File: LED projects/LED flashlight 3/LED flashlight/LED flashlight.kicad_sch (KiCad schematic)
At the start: 14 parts, among them P1 USB_C_Plug_USB2.0, SW1 SW_Push, U1 TP4056

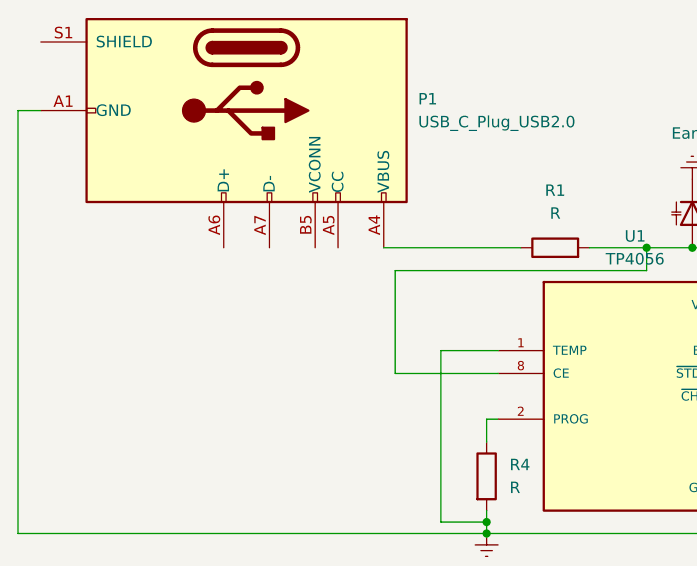
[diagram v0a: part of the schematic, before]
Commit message: update
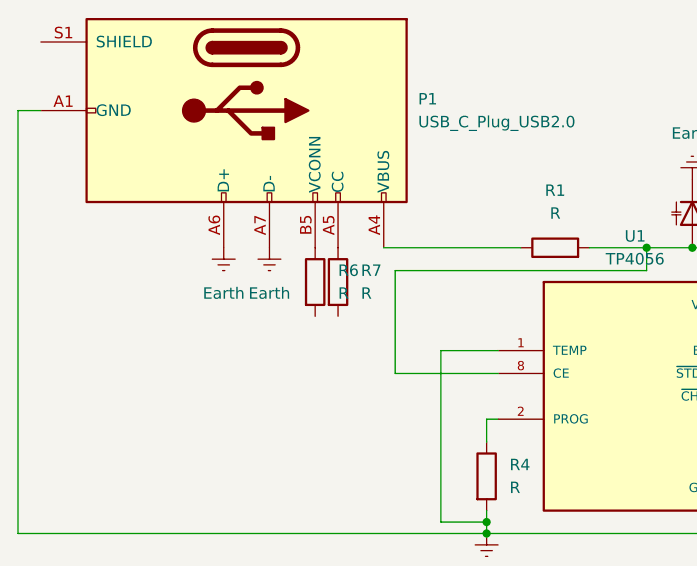
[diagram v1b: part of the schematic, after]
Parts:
- added R6, R7: R, symbol Device:R
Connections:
- net Earth: now also P1.A6 (D+), P1.A7 (D-)
- net at P1.A5 (CC): now also R7.1
- net at P1.B5 (VCONN): now also R6.1

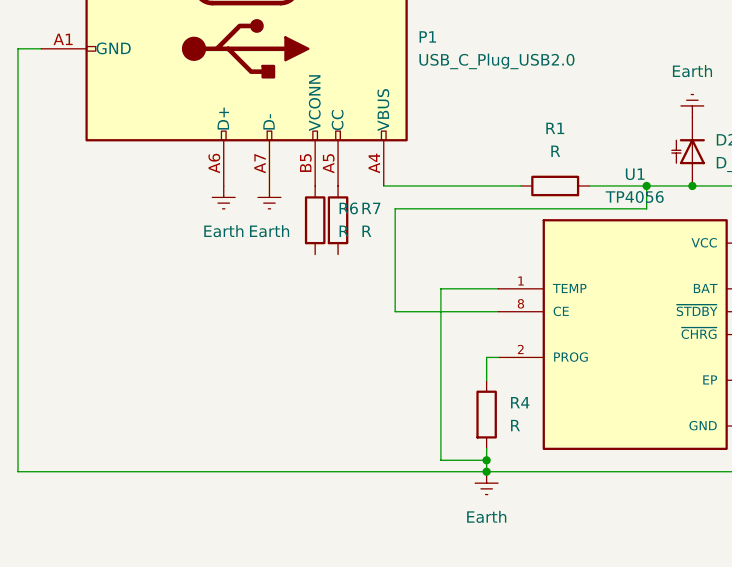
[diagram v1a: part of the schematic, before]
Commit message: update
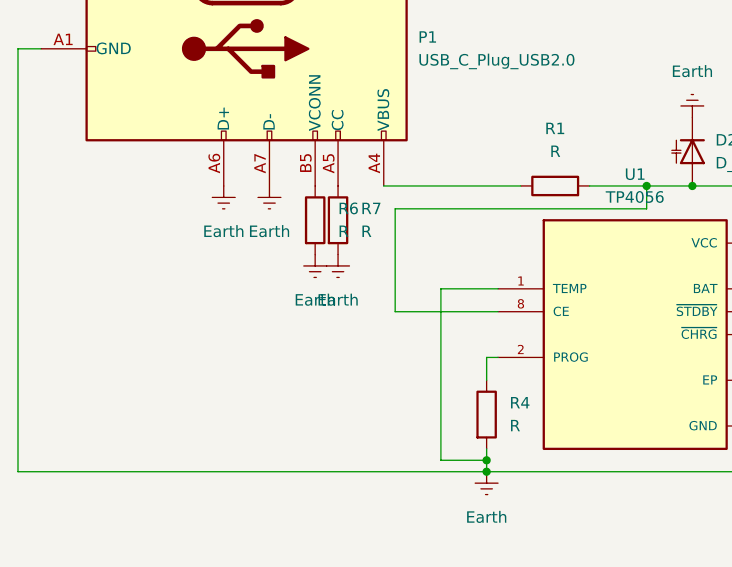
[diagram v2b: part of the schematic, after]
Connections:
- net Earth: now also R6.2, R7.2
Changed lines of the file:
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@@
+	)
+	(symbol
+		(lib_id "power:Earth")
+		(at 96.52 53.34 0)
+		(unit 1)
+		(exclude_from_sim no)
+		(in_bom yes)
+		(on_board yes)
+		(dnp no)
+		(fields_autoplaced yes)
+		(property "Reference" "#PWR07"
+			(at 96.52 59.69 0)
+			(effects
+				(font
+					(size 1.27 1.27)
+				)
+				(hide yes)
+			)
+		)
+		(property "Value" "Earth"
+			(at 96.52 58.42 0)
+			(effects
+				(font
+					(size 1.27 1.27)
+				)
+			)
+		)
+		(property "Footprint" ""
+			(at 96.52 53.34 0)
+			(effects
+				(font
+					(size 1.27 1.27)
+				)
+				(hide yes)
+			)
+		)
+		(property "Datasheet" "~"
+			(at 96.52 53.34 0)
+			(effects
+				(font
+					(size 1.27 1.27)
+				)
+				(hide yes)
+			)
+		)
+		(property "Description" "Power symbol creates a global label with name \"Earth\""
+			(at 96.52 53.34 0)
+			(effects
+				(font
+					(size 1.27 1.27)
+				)
+				(hide yes)
+			)
+		)
+		(pin "1"
+		)
+		(instances
+			(project "LED flashlight"
+				(path "/93811dea-1721-4415-96be-fa2e1cca3e57"
+					(reference "#PWR07")
+					(unit 1)
+				)
+			)
+		)
 	)
 	(symbol
@@
 					(unit 1)
 				)
+			)
+		)
+	)
+	(symbol
+		(lib_id "power:Earth")
+		(at 93.98 53.34 0)
+		(unit 1)
+		(exclude_from_sim no)
+		(in_bom yes)
+		(on_board yes)
+		(dnp no)
+		(fields_autoplaced yes)
+		(property "Reference" "#PWR06"
+			(at 93.98 59.69 0)
+			(effects
+				(font
+					(size 1.27 1.27)
+				)
+				(hide yes)
+			)
+		)
+		(property "Value" "Earth"
+			(at 93.98 58.42 0)
+			(effects
+				(font
+					(size 1.27 1.27)
+				)
+			)
+		)
+		(property "Footprint" ""
+			(at 93.98 53.34 0)
+			(effects
+				(font
+					(size 1.27 1.27)
+				)
+				(hide yes)
+			)
+		)
+		(property "Datasheet" "~"
+			(at 93.98 53.34 0)
+			(effects
+				(font
+					(size 1.27 1.27)
+				)
+				(hide yes)
+			)
+		)
+		(property "Description" "Power symbol creates a global label with name \"Earth\""
+			(at 93.98 53.34 0)
+			(effects
+				(font
+					(size 1.27 1.27)
+				)
+				(hide yes)
+			)
+		)
+		(pin "1"
+		)
+		(instances
+			(project "LED flashlight"
+				(path "/93811dea-1721-4415-96be-fa2e1cca3e57"
+					(reference "#PWR06")
+					(unit 1)
+				)
